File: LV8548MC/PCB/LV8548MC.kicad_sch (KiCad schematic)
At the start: 10 parts, among them J1 Conn_01x08_Socket, J2 Conn_01x02_Pin, J3 Conn_01x08_Pin, U1 LV8548MC, U2 LV8548MC, U4 L7805

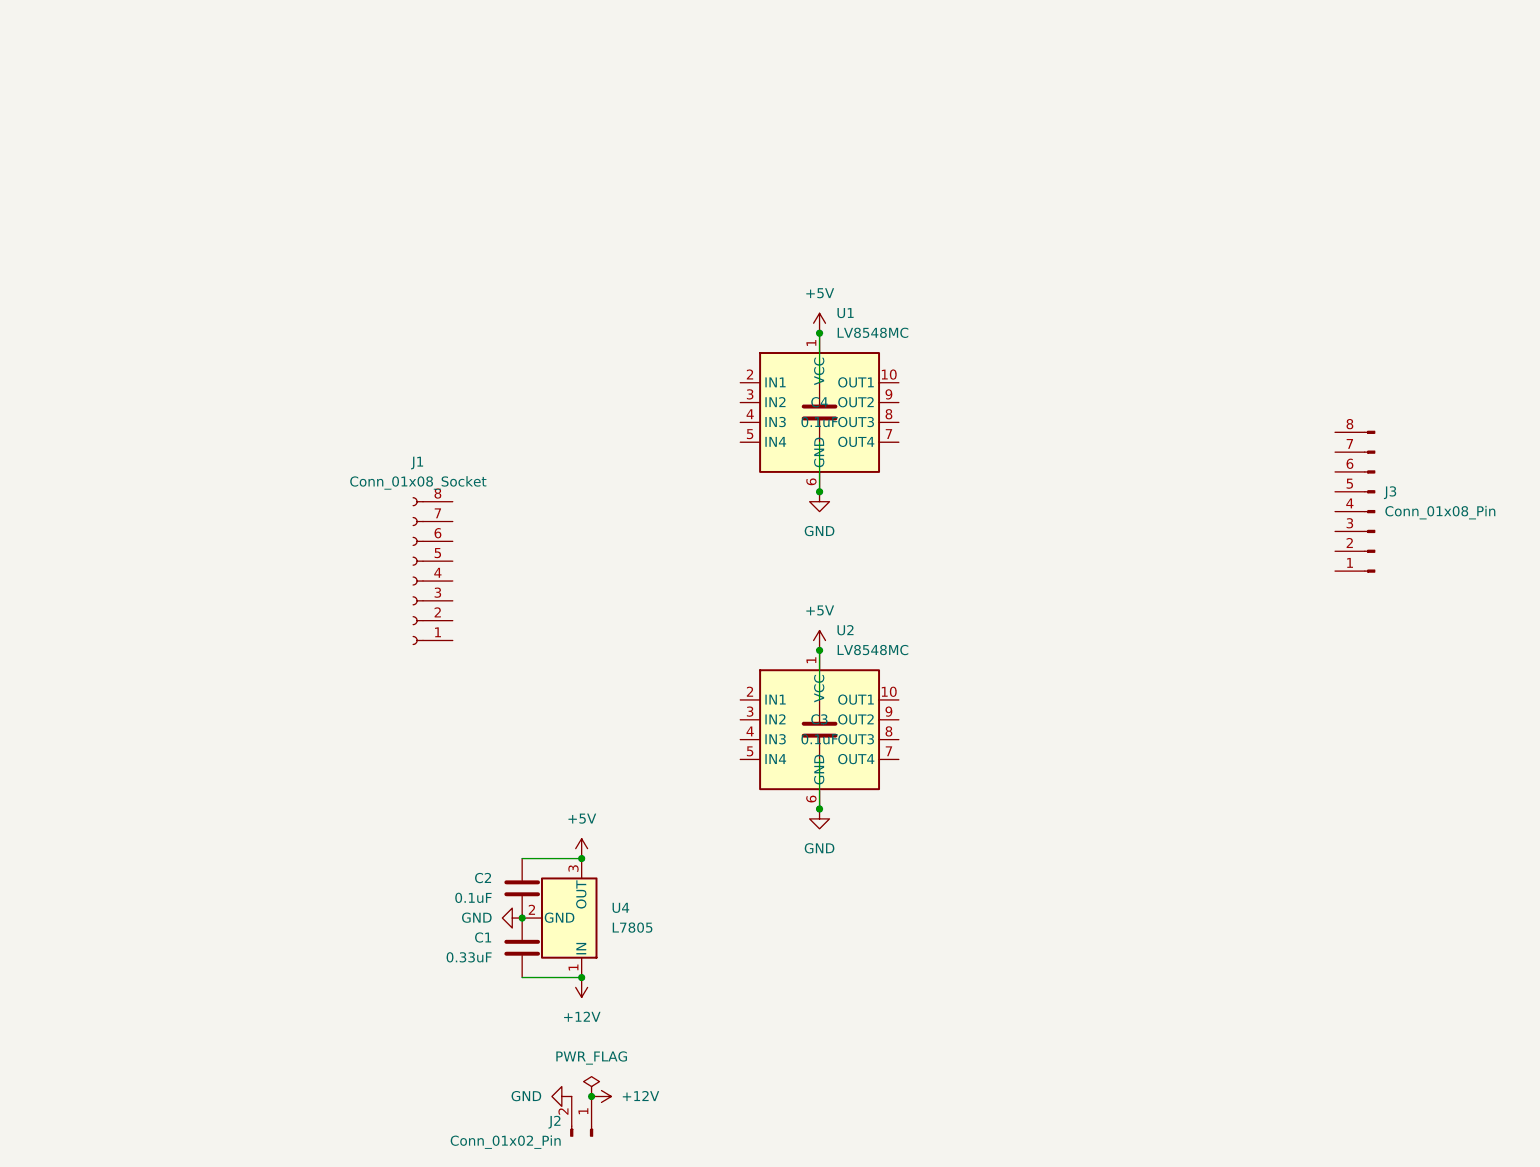
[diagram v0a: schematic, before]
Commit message: LV8548MC基板
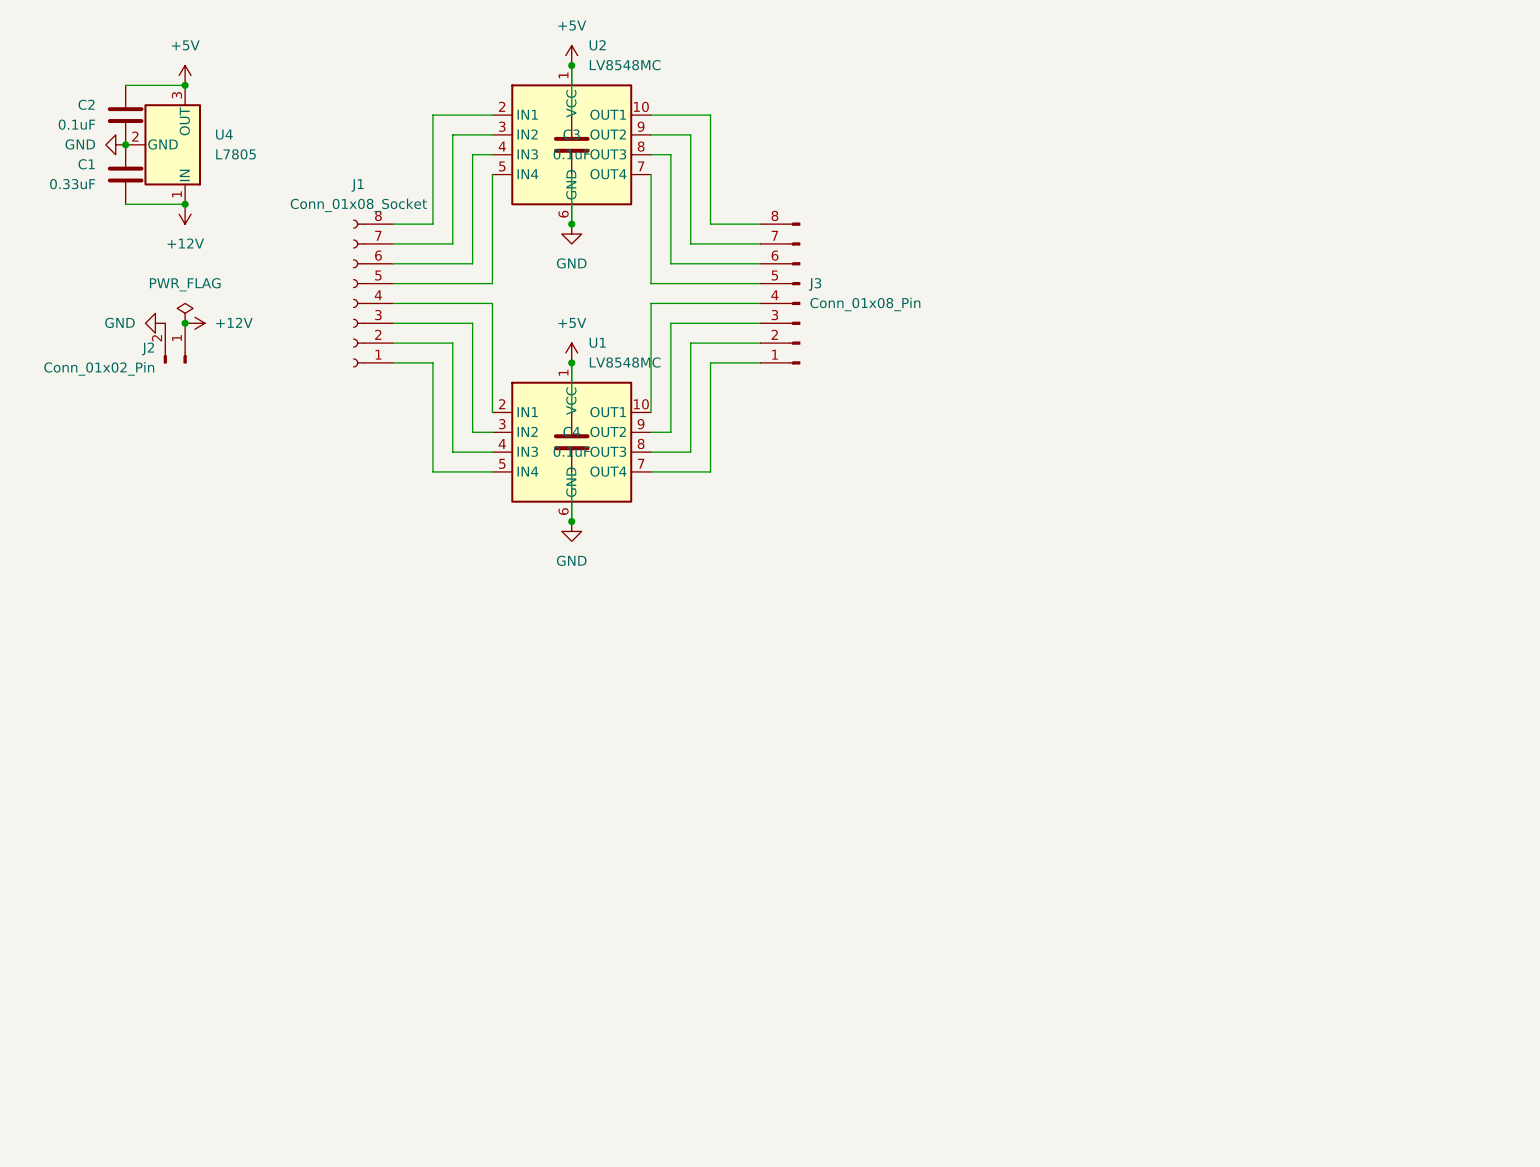
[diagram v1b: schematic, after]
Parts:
- U4: footprint Package_TO_SOT_THT:TO-220-3_Horizontal_TabUp -> Package_TO_SOT_THT:TO-220-3_Horizontal_TabDown
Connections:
- net at J3.1 (Pin_1): now also U1.7 (OUT4)
- net at J3.2 (Pin_2): now also U1.8 (OUT3)
- net at J3.3 (Pin_3): now also U1.9 (OUT2)
- net at J3.4 (Pin_4): now also U1.10 (OUT1)
- net at J3.5 (Pin_5): now also U2.7 (OUT4)
- net at J3.6 (Pin_6): now also U2.8 (OUT3)
- net at J3.7 (Pin_7): now also U2.9 (OUT2)
- net at J3.8 (Pin_8): now also U2.10 (OUT1)
- net at U1.2 (IN1): now also J1.4 (Pin_4)
- net at U1.3 (IN2): now also J1.3 (Pin_3)
- net at U1.4 (IN3): now also J1.2 (Pin_2)
- net at U1.5 (IN4): now also J1.1 (Pin_1)
- net at J1.5 (Pin_5): now also U2.5 (IN4)
- net at J1.6 (Pin_6): now also U2.4 (IN3)
- net at J1.7 (Pin_7): now also U2.3 (IN2)
- net at J1.8 (Pin_8): now also U2.2 (IN1)
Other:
- moved on the sheet: C1, C2, C3, C4, J1, J2, J3, U1, U2, U4
